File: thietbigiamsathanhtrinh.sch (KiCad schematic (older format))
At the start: 16 parts

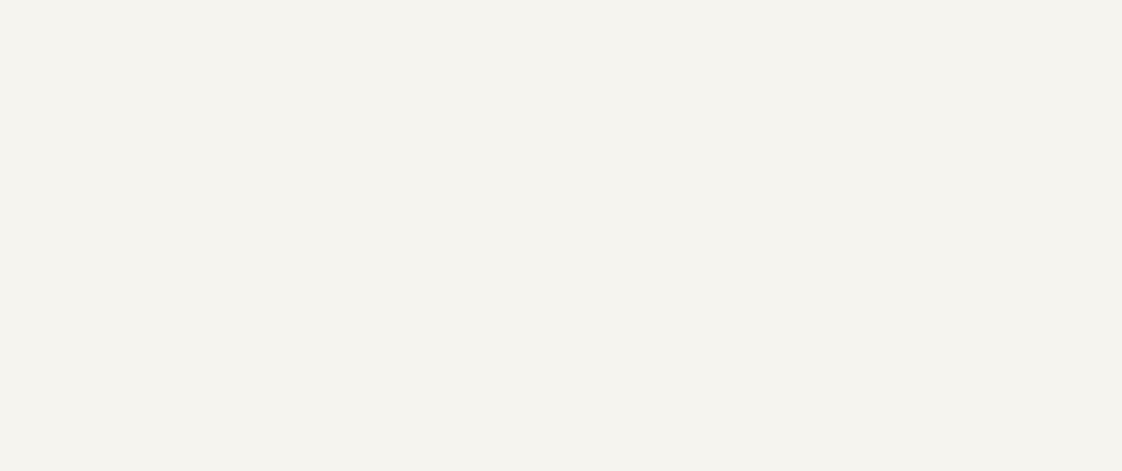
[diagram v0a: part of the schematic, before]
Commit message: lm8266
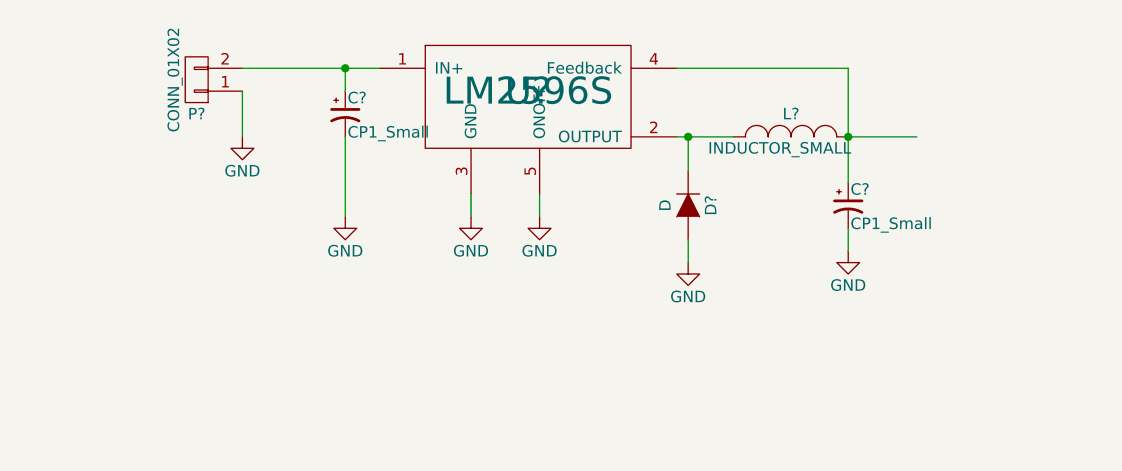
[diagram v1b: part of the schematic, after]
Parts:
- added C? (x2): CP1_Small, symbol CP1_Small
- added D?: D, symbol D
- added L?: INDUCTOR_SMALL, symbol INDUCTOR_SMALL
- added P?: CONN_01X02, symbol CONN_01X02
- added U?: LM2596S, symbol LM2596S
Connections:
- net GND: now also C?.2, C?.2, D?.2 (A), P?.1 (P1), U?.3 (GND), U?.5 (ONOFF)
- new net: C?.1, P?.2 (P2), U?.1 (IN+)
- new net: D?.1 (K), L?.1, U?.2 (OUTPUT)
- new net: C?.1, L?.2, U?.4 (Feedback)
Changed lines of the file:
@@
 LIBS:SIM800C
 LIBS:esp32-wrover-v3
+LIBS:lm2596s
+LIBS:thietbigiamsathanhtrinh-cache
 EELAYER 25 0
 EELAYER END
@@
 Wire Bus Line
 	5900 6000 500  6000
+$Comp
+L GND #PWR?
+U 1 1 59DC5B22
+P 8450 1350
+F 0 "#PWR?" H 8450 1100 50  0001 C CNN
+F 1 "GND" H 8450 1200 50  0000 C CNN
+F 2 "" H 8450 1350 50  0000 C CNN
+F 3 "" H 8450 1350 50  0000 C CNN
+	1    8450 1350
+	1    0    0    -1
+$EndComp
+$Comp
+L GND #PWR?
+U 1 1 59DC5BD7
+P 8150 1350
+F 0 "#PWR?" H 8150 1100 50  0001 C CNN
+F 1 "GND" H 8150 1200 50  0000 C CNN
+F 2 "" H 8150 1350 50  0000 C CNN
+F 3 "" H 8150 1350 50  0000 C CNN
+	1    8150 1350
+	1    0    0    -1
+$EndComp
+$Comp
+L CP1_Small C?
+U 1 1 59DC5C08
+P 7600 900
+F 0 "C?" H 7610 970 50  0000 L CNN
+F 1 "CP1_Small" H 7610 820 50  0000 L CNN
+F 2 "" H 7600 900 50  0000 C CNN
+F 3 "" H 7600 900 50  0000 C CNN
+	1    7600 900
+	1    0    0    -1
+$EndComp
+$Comp
+L D D?
+U 1 1 59DC5D21
+P 9100 1300
+F 0 "D?" H 9100 1400 50  0000 C CNN
+F 1 "D" H 9100 1200 50  0000 C CNN
+F 2 "" H 9100 1300 50  0000 C CNN
+F 3 "" H 9100 1300 50  0000 C CNN
+	1    9100 1300
+	0    1    1    0
+$EndComp
+$Comp
+L INDUCTOR_SMALL L?
+U 1 1 59DC5E3A
+P 9550 1000
+F 0 "L?" H 9550 1100 50  0000 C CNN
+F 1 "INDUCTOR_SMALL" H 9500 950 50  0000 C CNN
+F 2 "" H 9550 1000 50  0000 C CNN
+F 3 "" H 9550 1000 50  0000 C CNN
+	1    9550 1000
+	1    0    0    -1
+$EndComp
+$Comp
+L LM2596S U?
+U 1 1 59DC6476
+P 8400 800
+F 0 "U?" H 8400 800 118 0000 C CNN
+F 1 "LM2596S" H 8400 800 118 0000 C CNN
+F 2 "" H 8400 800 118 0000 C CNN
+F 3 "" H 8400 800 118 0000 C CNN
+	1    8400 800
+	1    0    0    -1
+$EndComp
+Wire Wire Line
+	7600 800  7600 700
+Wire Wire Line
+	7150 700  7750 700
+Wire Wire Line
+	9050 1000 9300 1000
+Wire Wire Line
+	9050 700  9800 700
+Wire Wire Line
+	9800 700  9800 1200
+Wire Wire Line
+	8150 1250 8150 1350
+Wire Wire Line
+	9100 1000 9100 1150
+Connection ~ 9100 1000
+$Comp
+L GND #PWR?
+U 1 1 59DC6C37
+P 9100 1550
+F 0 "#PWR?" H 9100 1300 50  0001 C CNN
+F 1 "GND" H 9100 1400 50  0000 C CNN
+F 2 "" H 9100 1550 50  0000 C CNN
+F 3 "" H 9100 1550 50  0000 C CNN
+	1    9100 1550
+	1    0    0    -1
+$EndComp
+Wire Wire Line
+	9100 1450 9100 1550
+Wire Wire Line
+	9800 1000 10100 1000
+Connection ~ 7600 700
+$Comp
+L GND #PWR?
+U 1 1 59DC6ECC
+P 7600 1350
+F 0 "#PWR?" H 7600 1100 50  0001 C CNN
+F 1 "GND" H 7600 1200 50  0000 C CNN
+F 2 "" H 7600 1350 50  0000 C CNN
+F 3 "" H 7600 1350 50  0000 C CNN
+	1    7600 1350
+	1    0    0    -1
+$EndComp
+Wire Wire Line
+	7600 1000 7600 1350
+Wire Wire Line
+	8450 1250 8450 1350
+$Comp
+L CP1_Small C?
+U 1 1 59DC718D
+P 9800 1300
+F 0 "C?" H 9810 1370 50  0000 L CNN
+F 1 "CP1_Small" H 9810 1220 50  0000 L CNN
+F 2 "" H 9800 1300 50  0000 C CNN
+F 3 "" H 9800 1300 50  0000 C CNN
+	1    9800 1300
+	1    0    0    -1
+$EndComp
+Connection ~ 9800 1000
+$Comp
+L GND #PWR?
+U 1 1 59DC72A4
+P 9800 1500
+F 0 "#PWR?" H 9800 1250 50  0001 C CNN
+F 1 "GND" H 9800 1350 50  0000 C CNN
+F 2 "" H 9800 1500 50  0000 C CNN
+F 3 "" H 9800 1500 50  0000 C CNN
+	1    9800 1500
+	1    0    0    -1
+$EndComp
+Wire Wire Line
+	9800 1400 9800 1500
+$Comp
+L CONN_01X02 P?
+U 1 1 59DC73F4
+P 6950 750
+F 0 "P?" H 6950 900 50  0000 C CNN
+F 1 "CONN_01X02" V 7050 750 50  0000 C CNN
+F 2 "" H 6950 750 50  0000 C CNN
+F 3 "" H 6950 750 50  0000 C CNN
+	1    6950 750
+	-1   0    0    1
+$EndComp
+$Comp
+L GND #PWR?
+U 1 1 59DC7563
+P 7150 1000
+F 0 "#PWR?" H 7150 750 50  0001 C CNN
+F 1 "GND" H 7150 850 50  0000 C CNN
+F 2 "" H 7150 1000 50  0000 C CNN
+F 3 "" H 7150 1000 50  0000 C CNN
+	1    7150 1000
+	1    0    0    -1
+$EndComp
+Wire Wire Line
+	7150 800  7150 1000
 $EndSCHEMATC
